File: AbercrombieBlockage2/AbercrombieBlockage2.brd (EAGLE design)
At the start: 38 x 38 mm, 35 parts, among them U1 DMN3135LVT, U2 ICS-43434, U3 CYBLE-022001-00, U4 LIS3DH, U5 VL53L0X, U6 VL53L0X, U7 VL53L0X, U8 M24

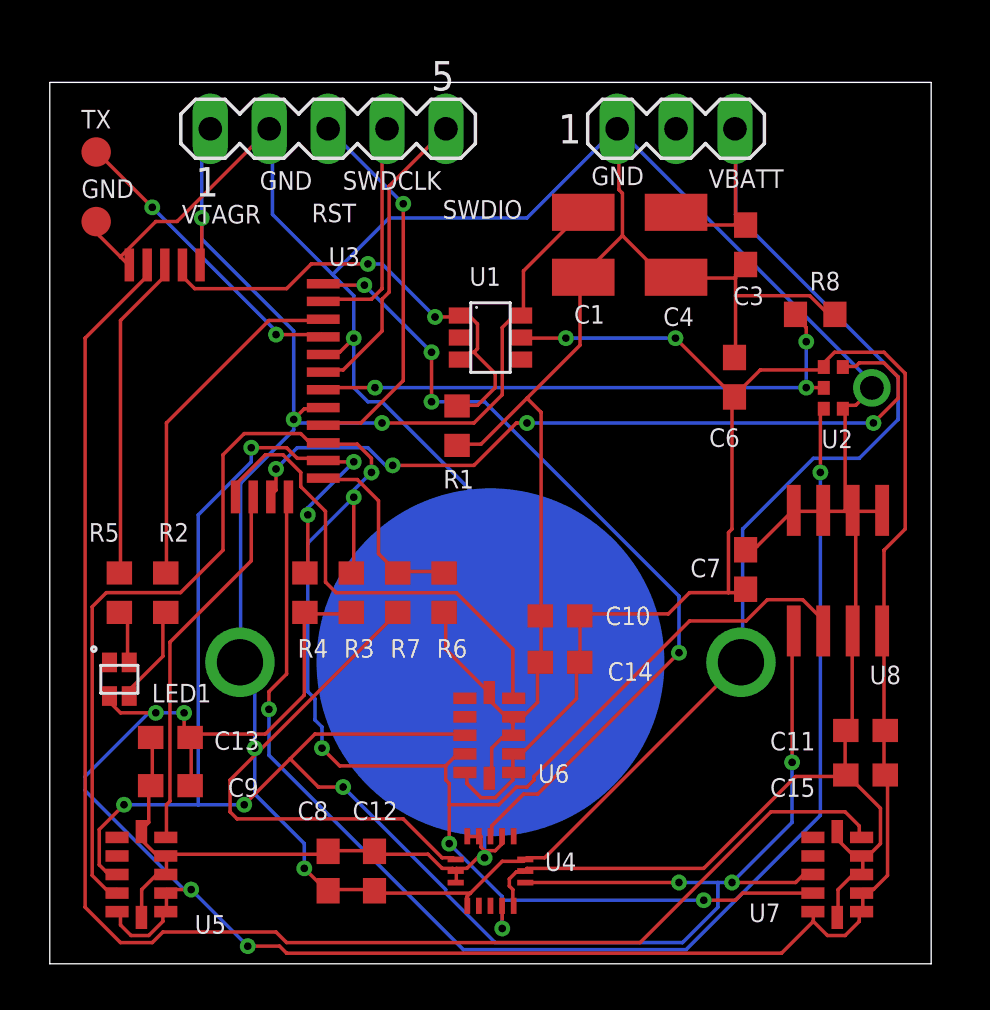
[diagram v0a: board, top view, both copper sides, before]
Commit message: Routed the Abercrombie Laser project.
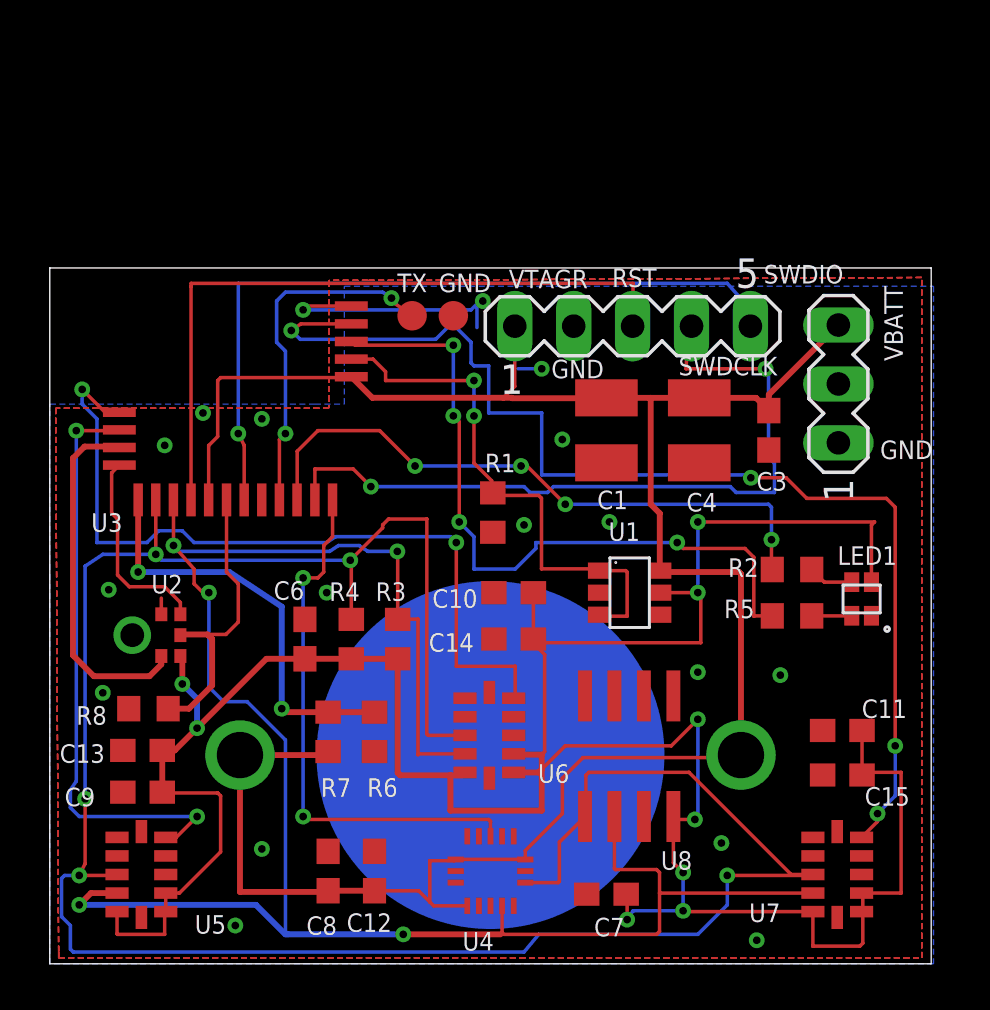
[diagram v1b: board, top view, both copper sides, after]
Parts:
- moved R8 33.4 mm to (4.25, 11.0), turned to 180 degrees
- moved LED1 32.2 mm to (35.0, 15.7), turned to 180 degrees
- moved U2 29.7 mm to (5.63, 14.2), turned to 180 degrees
- moved R5 29.0 mm to (32.0, 15.0), turned to 180 degrees
- moved R2 27.0 mm to (32.0, 17.0), turned to 180 degrees
- moved C6 21.7 mm to (11.0, 14.0)
- moved GND 15.9 mm to (17.4, 27.9)
- moved SV2 15.6 mm to (25.1, 27.5)
- moved TX 15.3 mm to (15.6, 27.9)
- moved C7 15.2 mm to (24.0, 3.00), turned to 180 degrees
- moved SV1 13.0 mm to (34.0, 25.0), turned to 90 degrees
- moved U1 12.5 mm to (25.0, 16.0)
- moved U8 12.0 mm to (25.0, 8.95)
- moved C1 8.06 mm to (24.0, 23.0)
- moved C3 8.06 mm to (31.0, 23.0)
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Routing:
- net GND: track 214.3 -> 13.1 mm, vias 2 -> 18
- net WS: track 58.8 -> 8.69 mm, vias 2 -> 0
- net VDD: track 142.5 -> 95.0 mm, vias 5 -> 0
- net SWDCLK: track 9.75 -> 33.5 mm, vias 0 -> 2
- net SWDIO: track 13.1 -> 32.7 mm, vias 0 -> 1
- net SCK: track 33.6 -> 15.5 mm, vias 4 -> 0
- net GREEN_LED: track 14.1 -> 30.8 mm, vias 0 -> 4
- net XSHUT_3: track 66.3 -> 50.5 mm, vias 0 -> 4
- net V+: track 138.3 -> 122.8 mm, vias 6 -> 9
- net XRES: track 16.4 -> 30.2 mm, vias 1 -> 0
- net XSHUT_2: track 20.7 -> 34.3 mm, vias 0 -> 2
- net SCL: track 98.2 -> 85.2 mm, vias 6 -> 5
- net WAKEUP: track 36.2 -> 23.4 mm, vias 4 -> 2
- net SDI: track 25.0 -> 12.8 mm, vias 3 -> 0
- net BLUE_LED: track 15.1 -> 27.0 mm, vias 0 -> 4
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- added copper zone on layer 1, net GND
- added copper zone on layer 16, net GND
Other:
- board size 38 x 38 mm -> 38 x 30 mm
